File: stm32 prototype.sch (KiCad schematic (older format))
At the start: 132 parts, among them J1 USB_B_Mini, J2 Conn_01x06, J3 Conn_01x02, Q1 Q_NMOS_GSD, Q2 Q_NMOS_GSD, Q3 Q_NMOS_GSD, Q4 Q_NMOS_GSD, Q5 Q_NMOS_GSD, Q6 Q_NMOS_GSD, Q7 Q_NMOS_GSD, Q8 Q_NMOS_GSD, Q9 Q_NMOS_GSD, U1 FT232RL, U2 W25Q128JV-DTR, U3 STM32F407VGTx, U4 LD1117S33TR, U5 ESP32, U6 IS25LP016D-JNLE-TR, U7 TPS62203DBVR, Y1 Crystal_GND24, Y2 Crystal_GND23, Y3 Crystal_GND23

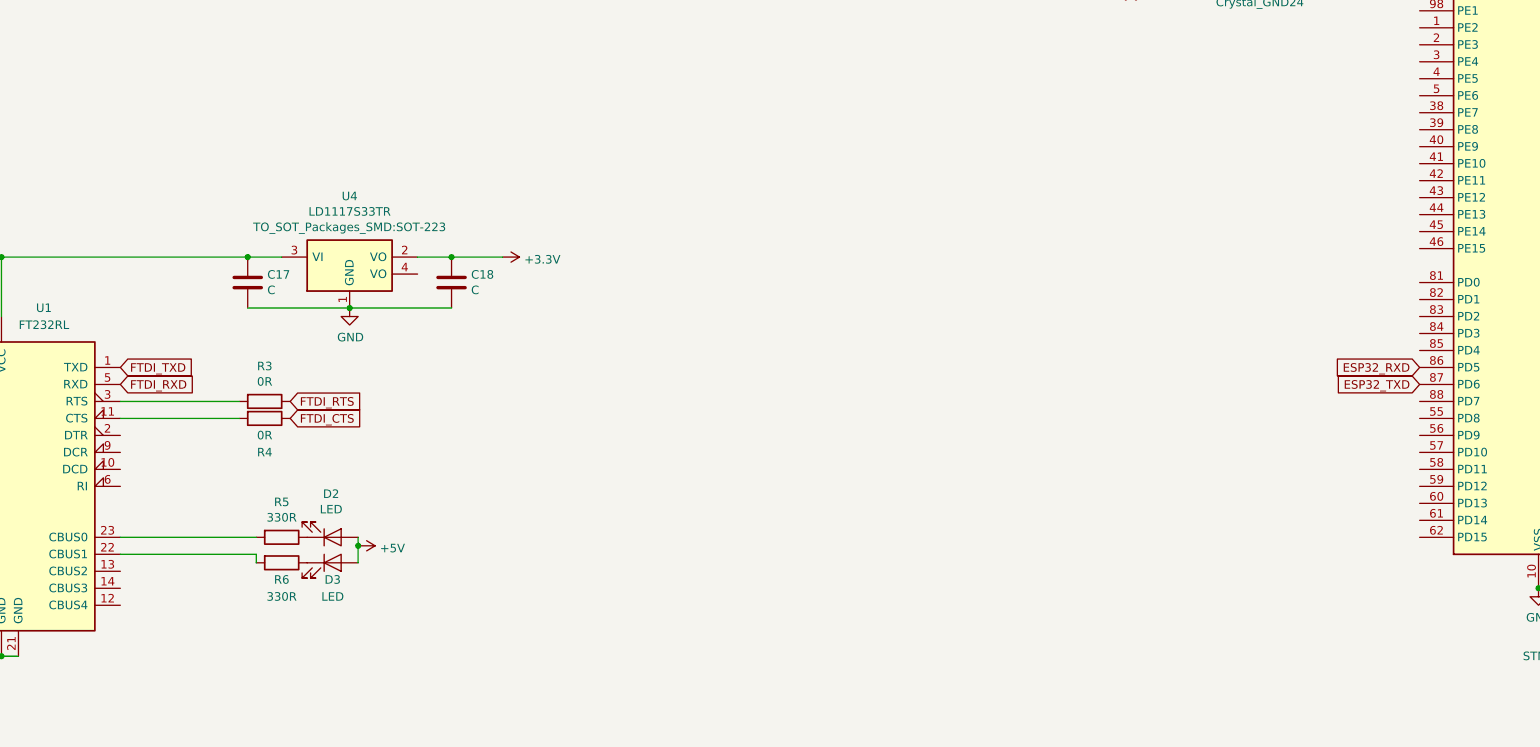
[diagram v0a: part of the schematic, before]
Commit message: worked on some layout around the stm32f
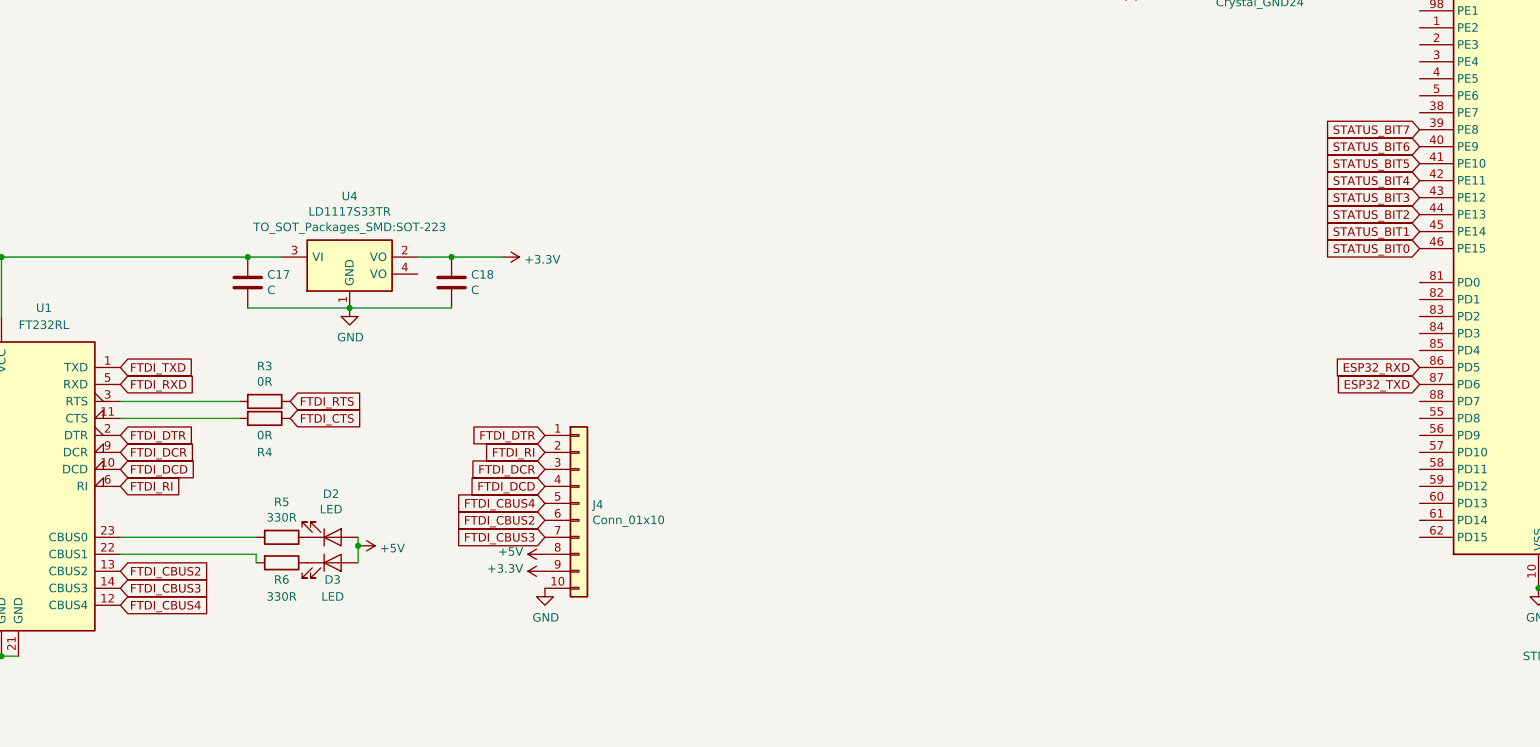
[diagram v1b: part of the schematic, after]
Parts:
- added J4: Conn_01x10, Pin_Headers:Pin_Header_Straight_1x10_Pitch2.54mm, symbol Connector_Generic:Conn_01x10
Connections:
- net +3V3: now also J4.9 (Pin_9)
- net +5V: now also J4.8 (Pin_8)
- net GND: now also J4.10 (Pin_10)
- net STATUS_BIT0: now also U3.46 (PE15)
- net STATUS_BIT1: now also U3.45 (PE14)
- net STATUS_BIT2: now also U3.44 (PE13)
- net STATUS_BIT3: now also U3.43 (PE12)
- net STATUS_BIT4: now also U3.42 (PE11)
- net STATUS_BIT5: now also U3.41 (PE10)
- net STATUS_BIT6: now also U3.40 (PE9)
- net STATUS_BIT7: now also U3.39 (PE8)
- net FTDI_DCD: now reaches U1.10 (DCD)
- net FTDI_DCD: now also J4.4 (Pin_4)
- net FTDI_CBUS4: now reaches U1.12 (CBUS4)
- net FTDI_CBUS4: now also J4.5 (Pin_5)
- net FTDI_CBUS2: now reaches U1.13 (CBUS2)
- net FTDI_CBUS2: now also J4.6 (Pin_6)
- net FTDI_CBUS3: now reaches U1.14 (CBUS3)
- net FTDI_CBUS3: now also J4.7 (Pin_7)
- net FTDI_DTR: now reaches U1.2 (DTR)
- net FTDI_DTR: now also J4.1 (Pin_1)
- net FTDI_RI: now reaches U1.6 (RI)
- net FTDI_RI: now also J4.2 (Pin_2)
- net FTDI_DCR: now reaches U1.9 (DCR)
- net FTDI_DCR: now also J4.3 (Pin_3)
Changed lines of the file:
@@
 Text Notes 2200 6300 0    79   ~ 0
 POWER OK LEDS
+Text GLabel 14450 8650 0    50   Input ~ 0
+STATUS_BIT0
+Text GLabel 14450 8550 0    50   Input ~ 0
+STATUS_BIT1
+Text GLabel 14450 8450 0    50   Input ~ 0
+STATUS_BIT2
+Text GLabel 14450 8350 0    50   Input ~ 0
+STATUS_BIT3
+Text GLabel 14450 8250 0    50   Input ~ 0
+STATUS_BIT4
+Text GLabel 14450 8150 0    50   Input ~ 0
+STATUS_BIT5
+Text GLabel 14450 8050 0    50   Input ~ 0
+STATUS_BIT6
+Text GLabel 14450 7950 0    50   Input ~ 0
+STATUS_BIT7
+$Comp
+L Connector_Generic:Conn_01x10 J4
+U 1 1 5C3119D0
+P 9500 10150
+F 0 "J4" H 9580 10142 50  0000 L CNN
+F 1 "Conn_01x10" H 9580 10051 50  0000 L CNN
+F 2 "Pin_Headers:Pin_Header_Straight_1x10_Pitch2.54mm" H 9500 10150 50  0001 C CNN
+F 3 "~" H 9500 10150 50  0001 C CNN
+	1    9500 10150
+	1    0    0    -1
+$EndComp
+Text GLabel 6800 9750 2    50   Input ~ 0
+FTDI_DTR
+Text GLabel 6800 9850 2    50   Input ~ 0
+FTDI_DCR
+Text GLabel 6800 9950 2    50   Input ~ 0
+FTDI_DCD
+Text GLabel 6800 10050 2    50   Input ~ 0
+FTDI_RI
+Text GLabel 6800 10550 2    50   Input ~ 0
+FTDI_CBUS2
+Text GLabel 6800 10650 2    50   Input ~ 0
+FTDI_CBUS3
+Text GLabel 6800 10750 2    50   Input ~ 0
+FTDI_CBUS4
+Text GLabel 9300 9750 0    50   Input ~ 0
+FTDI_DTR
+Text GLabel 9300 9850 0    50   Input ~ 0
+FTDI_RI
+Text GLabel 9300 9950 0    50   Input ~ 0
+FTDI_DCR
+Text GLabel 9300 10050 0    50   Input ~ 0
+FTDI_DCD
+Text GLabel 9300 10150 0    50   Input ~ 0
+FTDI_CBUS4
+Text GLabel 9300 10250 0    50   Input ~ 0
+FTDI_CBUS2
+Text GLabel 9300 10350 0    50   Input ~ 0
+FTDI_CBUS3
+$Comp
+L power:+5V #PWR0155
+U 1 1 5C3158AD
+P 9300 10450
+F 0 "#PWR0155" H 9300 10300 50  0001 C CNN
+F 1 "+5V" V 9315 10578 50  0000 L CNN
+F 2 "" H 9300 10450 50  0001 C CNN
+F 3 "" H 9300 10450 50  0001 C CNN
+	1    9300 10450
+	0    -1   -1   0
+$EndComp
+$Comp
+L power:+3.3V #PWR0156
+U 1 1 5C315DEA
+P 9300 10550
+F 0 "#PWR0156" H 9300 10400 50  0001 C CNN
+F 1 "+3.3V" V 9315 10678 50  0000 L CNN
+F 2 "" H 9300 10550 50  0001 C CNN
+F 3 "" H 9300 10550 50  0001 C CNN
+	1    9300 10550
+	0    -1   -1   0
+$EndComp
+$Comp
+L power:GND #PWR0157
+U 1 1 5C316BFC
+P 9300 10650
+F 0 "#PWR0157" H 9300 10400 50  0001 C CNN
+F 1 "GND" H 9305 10477 50  0000 C CNN
+F 2 "" H 9300 10650 50  0001 C CNN
+F 3 "" H 9300 10650 50  0001 C CNN
+	1    9300 10650
+	1    0    0    -1
+$EndComp
 $EndSCHEMATC
